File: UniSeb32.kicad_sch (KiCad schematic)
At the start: 35 parts

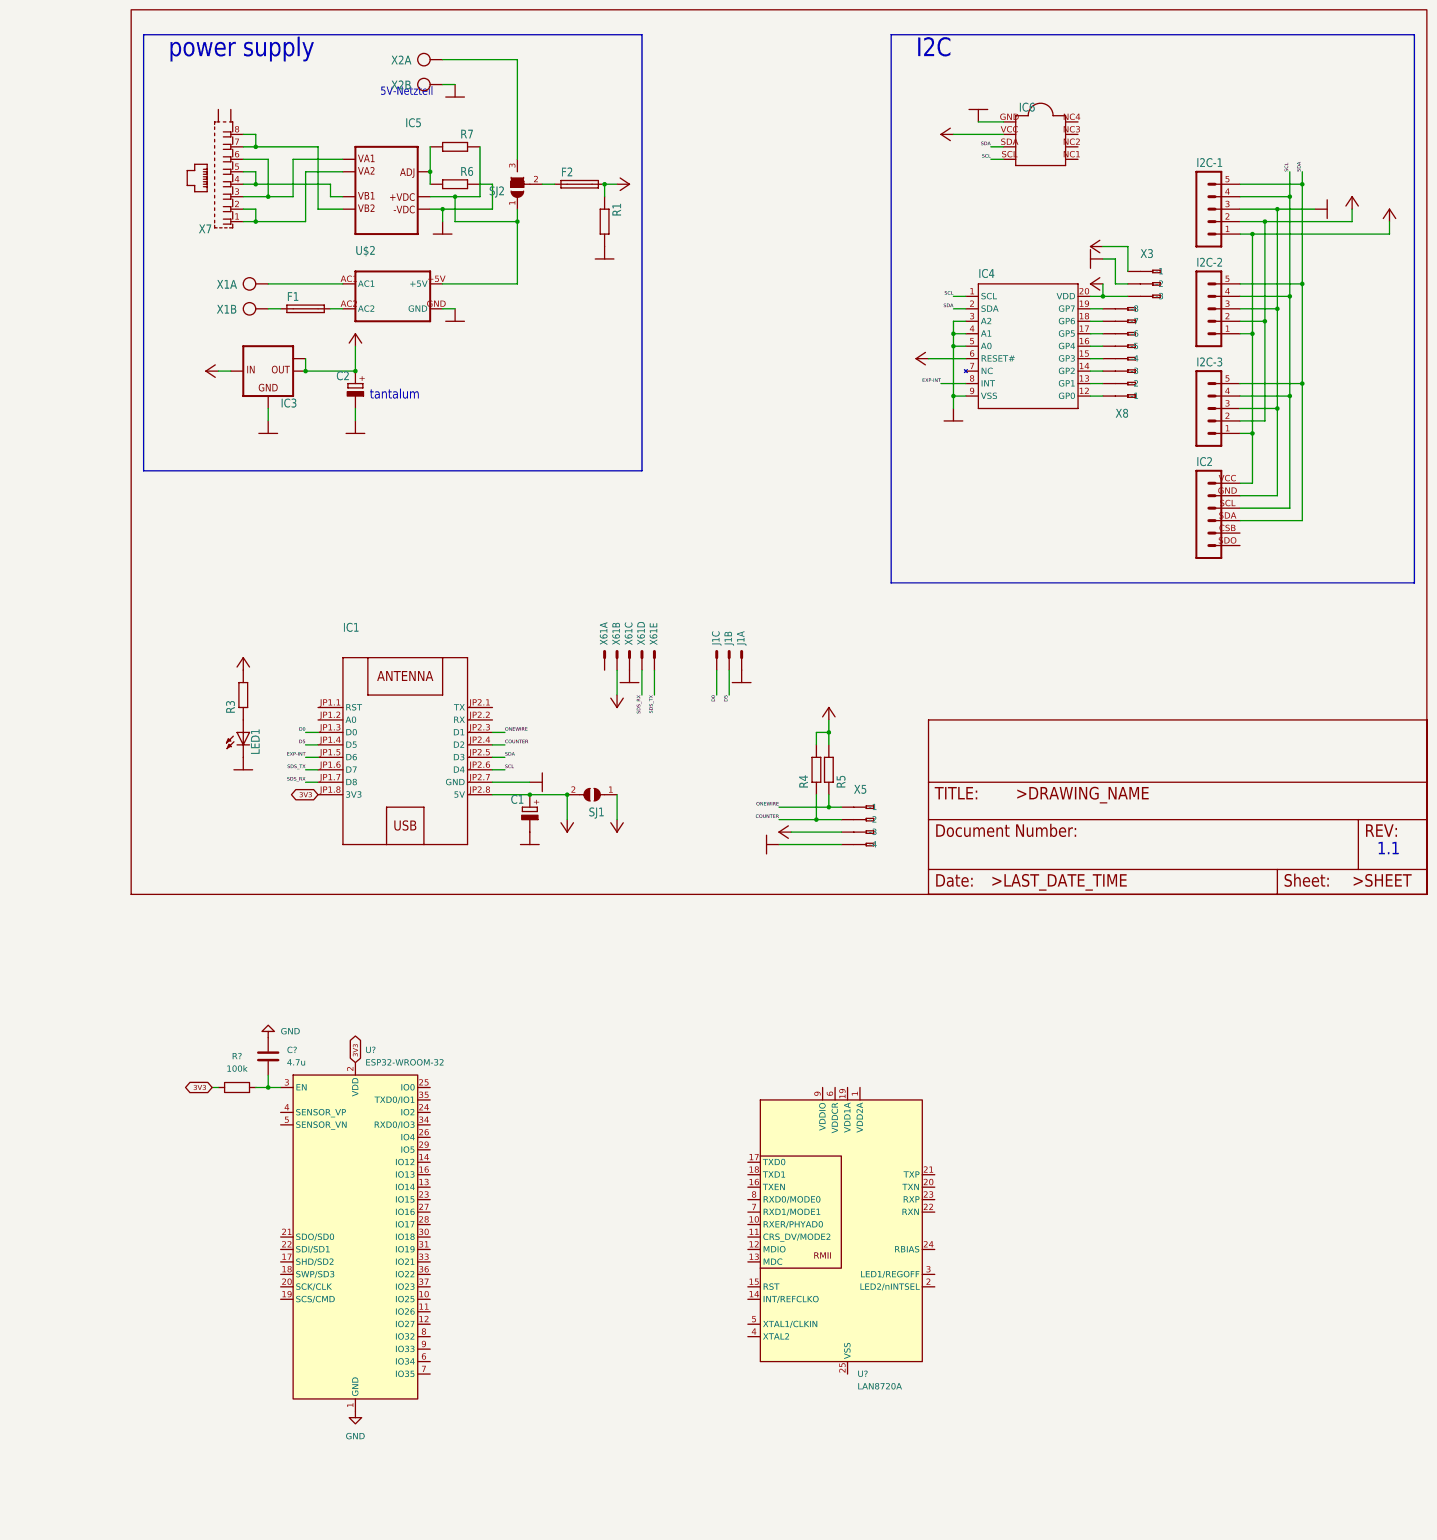
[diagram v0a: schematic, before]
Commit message: -
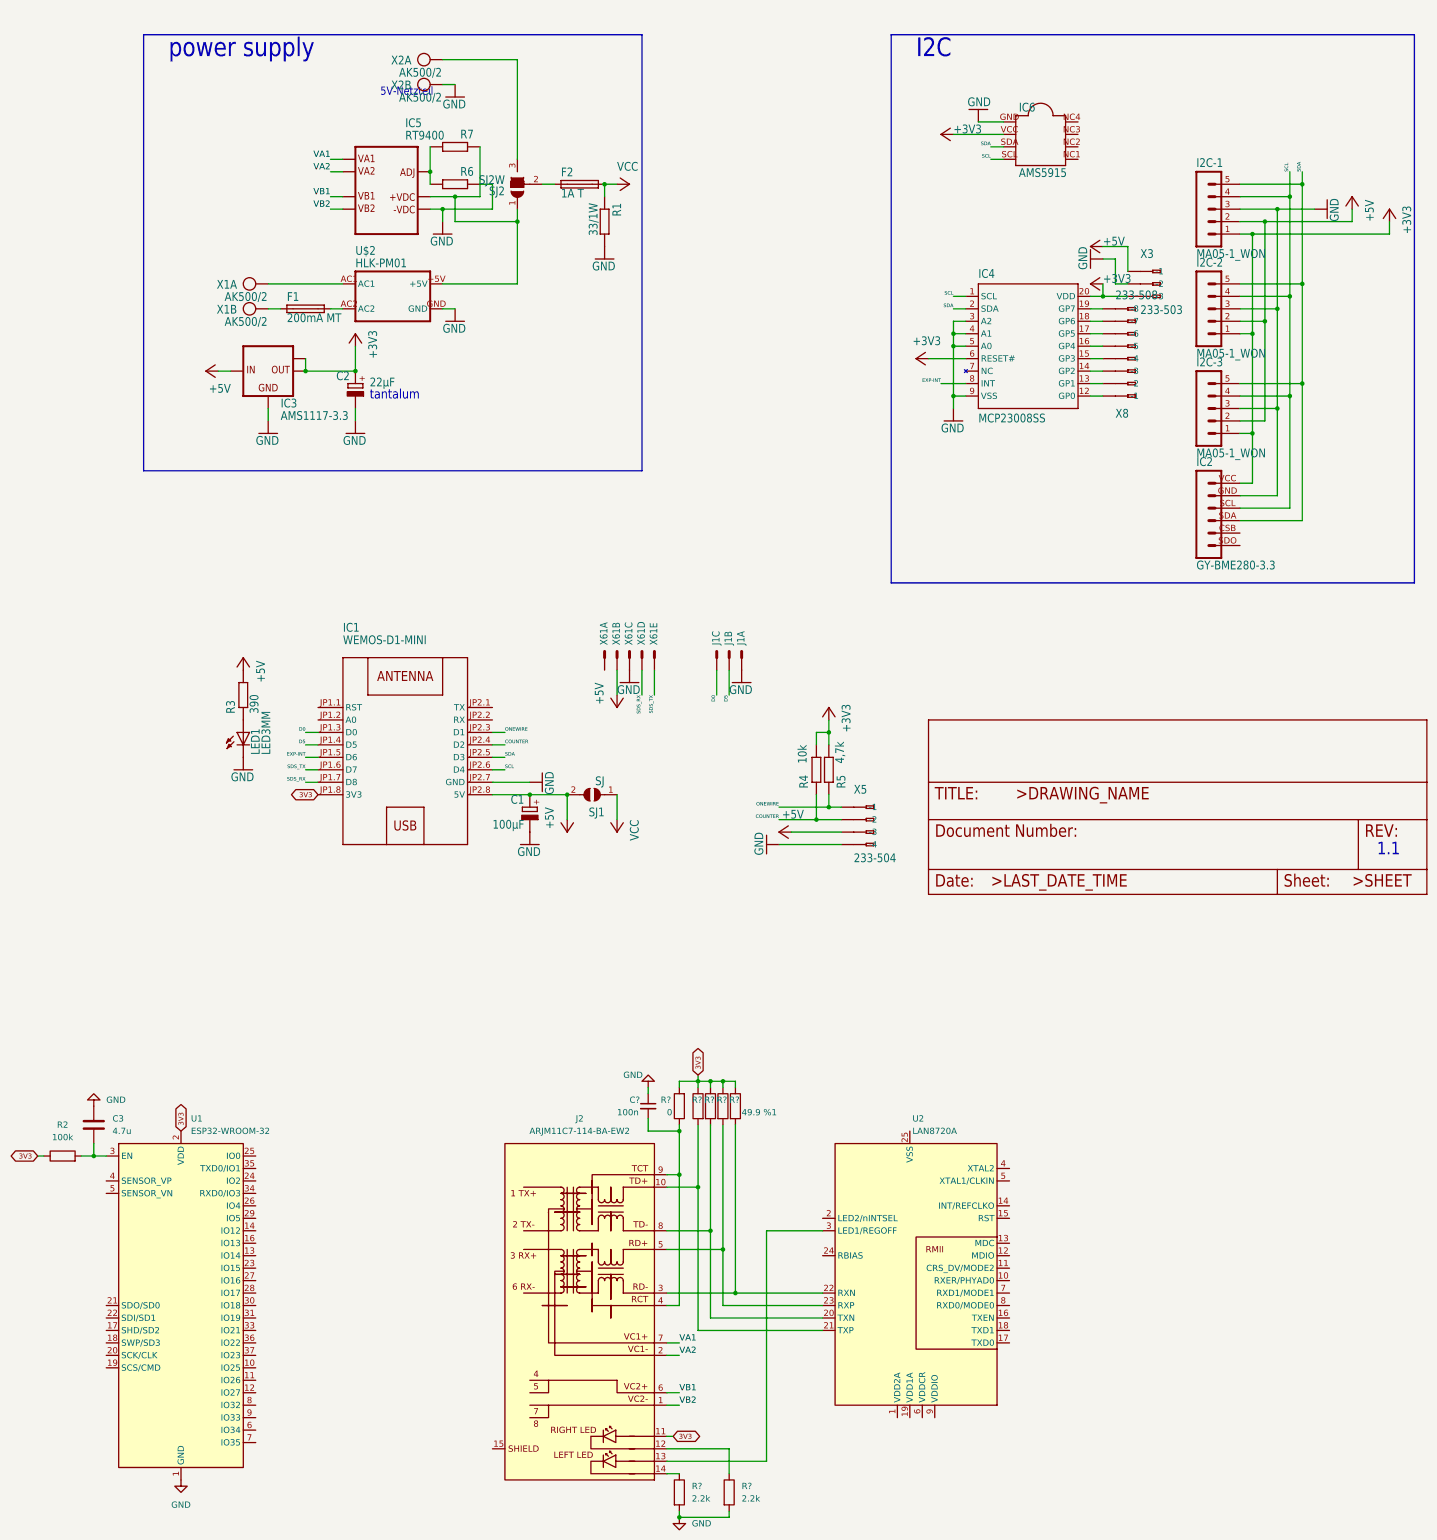
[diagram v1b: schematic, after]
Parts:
- removed X7: (no value), symbol UniSeb8266-eagle-import:0446200002
- added C?: 100n, symbol Device:C_Small
- added J2: ARJM11C7-114-BA-EW2, Connector_RJ:RJ45_Abracon_ARJM11C-BA, symbol Connector-custom:RJ45_Abracon_ARJM11C7-114
- added R? (x2): 2.2k, Resistor_SMD:R_0603_1608Metric, symbol Device:R
- added R? (x4): 49.9 %1, Resistor_SMD:R_0603_1608Metric, symbol Device:R
- added R?: 0, Resistor_SMD:R_0603_1608Metric, symbol Device:R
- C1: value (none) -> 100µF; footprint (none) -> UniSeb8266:E2,5-6
- C2: value (none) -> 22µF; footprint (none) -> UniSeb8266:E2,5-6
- F1: value (none) -> 200mA MT; footprint (none) -> UniSeb8266:TR5
- F2: value (none) -> 1A T; footprint (none) -> UniSeb8266:TR5
- I2C-1, I2C-2, I2C-3: value (none) -> MA05-1_WON; footprint (none) -> UniSeb8266:MA05-1_WON
- IC1: value (none) -> WEMOS-D1-MINI; footprint (none) -> UniSeb8266:WEMOS-D1-MINI
- IC2: value (none) -> GY-BME280-3.3; footprint (none) -> UniSeb8266:GY-BME280-3.3
- IC3: value (none) -> AMS1117-3.3; footprint (none) -> UniSeb8266:SOT223
- IC4: value (none) -> MCP23008SS; footprint (none) -> UniSeb8266:SSOP20
- IC5: value (none) -> RT9400; footprint (none) -> UniSeb8266:RT9400
- IC6: value (none) -> AMS5915; footprint (none) -> UniSeb8266:AMS5915
- J1: value (none) -> 22-?-0327-2031; footprint (none) -> UniSeb8266:6410-03
- LED1: value (none) -> LED3MM; footprint (none) -> UniSeb8266:LED3MM
- R1: value (none) -> 33/1W; footprint (none) -> UniSeb8266:P0613V
- R2: renamed from R?; footprint (none) -> Resistor_SMD:R_0603_1608Metric
- R3: value (none) -> 390; footprint (none) -> UniSeb8266:R1206
- R4: value (none) -> 10k; footprint (none) -> UniSeb8266:R1206
- R5: value (none) -> 4,7k; footprint (none) -> UniSeb8266:R1206
- R6, R7: value (none) -> R-EU_R1206; footprint (none) -> UniSeb8266:R1206
- SJ1: value (none) -> SJ; footprint (none) -> UniSeb8266:SJ
- SJ2: value (none) -> SJ2W; footprint (none) -> UniSeb8266:SJ_2
- U$2: value (none) -> HLK-PM01; footprint (none) -> UniSeb8266:HLK-PM01
- X1, X2: value (none) -> AK500/2; footprint (none) -> UniSeb8266:AK500_2
- X3: value (none) -> 233-503; footprint (none) -> UniSeb8266:233-503
- X5: value (none) -> 233-504; footprint (none) -> UniSeb8266:233-504
- X61: value (none) -> JST-XH-05-PIN-LONG-PAD; footprint (none) -> UniSeb8266:JST-XH-05-PACKAGE-LONG-PAD
- X8: value (none) -> 233-508; footprint (none) -> UniSeb8266:233-508
- gave numbers to parts that had none: 3
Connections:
- net 3V3: now also J2.11 (RLED+), R?.1, R?.1, R?.1, R?.1, R?.2
- net GND: now also C?.1, R?.2, R?.2
- net at U2.20 (TXN): now also J2.8 (TD-), R?.2
- net at U2.21 (TXP): now also J2.10 (TD+), R?.2
- net at U2.22 (RXN): now also J2.3 (RD-), R?.2
- net at U2.23 (RXP): now also J2.5 (RD+), R?.2
- net at U2.3 (LED1/REGOFF): now also J2.13 (LLED+)
- net VA2: now reaches IC5.P$2 (VA2)
- net VA2: now also J2.2 (VC1-)
- net VA1: now reaches IC5.P$1 (VA1)
- net VA1: now also J2.7 (VC1+)
- net VB1: now reaches IC5.P$3 (VB1)
- net VB1: now also J2.6 (VC2+)
- net VB2: now reaches IC5.P$4 (VB2)
- net VB2: now also J2.1 (VC2-)
- new net: J2.12 (RLED-), R?.1
- new net: J2.14 (LLED-), R?.1
- new net: C?.2, J2.4 (RCT), J2.9 (TCT), R?.1
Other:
- moved on the sheet: C3, R2, U1, U2
